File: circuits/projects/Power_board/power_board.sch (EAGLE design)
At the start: 5 parts

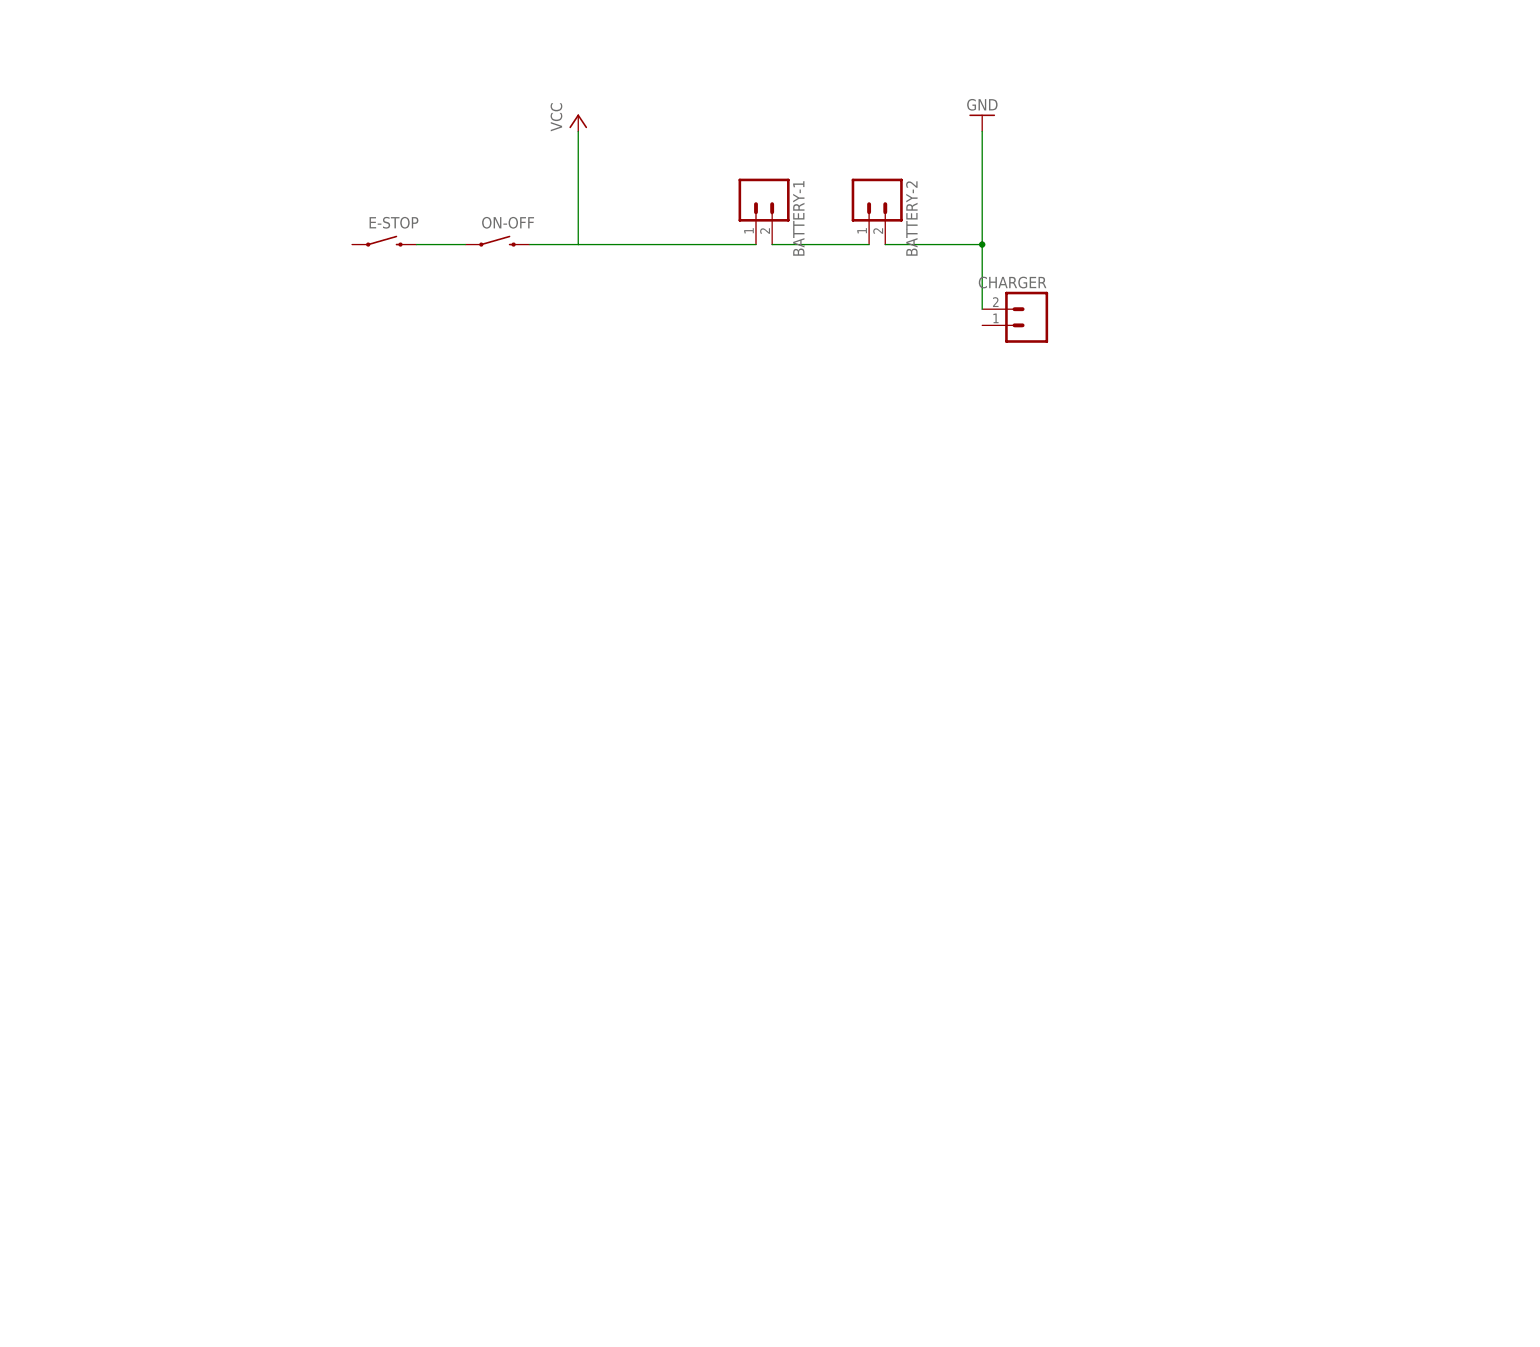
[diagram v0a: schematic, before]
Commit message: circuit board work
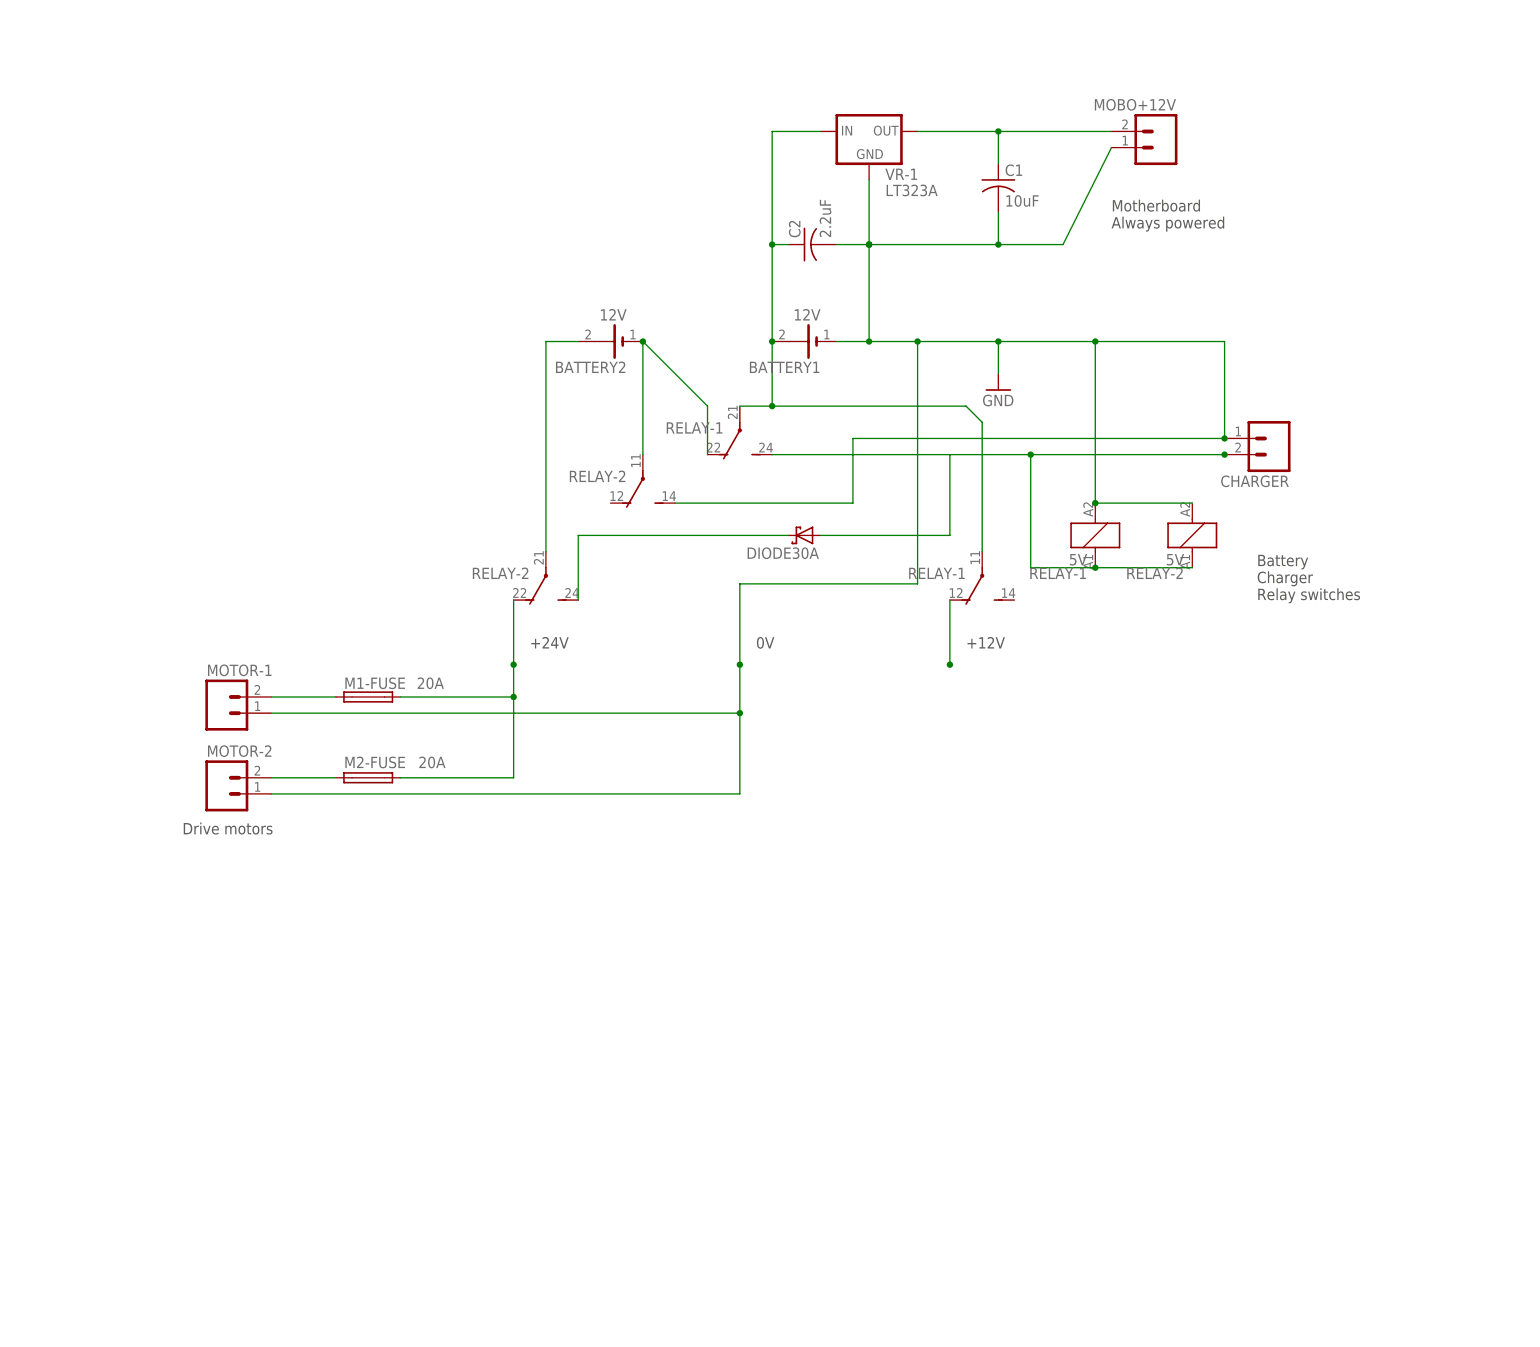
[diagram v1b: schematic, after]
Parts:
- removed BATTERY-1, BATTERY-2: (no value), iStivi - Header-Connector:M02-1.5MM
- removed E-STOP, ON-OFF: 2-PIN-SWITCH2X1.5MM_HOLES, iStivi - Button-Switch:2-PIN-SWITCH2X1.5MM_HOLES
- added BATTERY1, BATTERY2: 12V, parts:BATTERY-ST
- added C1: 10uF, parts:CAPACITOR
- added C2: 2.2uF, parts:CAPACITOR
- added DIODE30A: NTST30100SG-H, parts:NTST30100SG-H
- added M1-FUSE, M2-FUSE: 20A, parts:FUSE
- added MOBO+12V: 2-HOLESSC3.81MM, parts:2-HOLESSC3.81MM
- added MOTOR-1, MOTOR-2: 2-HOLESSC5MM, parts:2-HOLESSC5MM
- added RELAY-1, RELAY-2: 5V, parts:RT424A05
- added VR-1: LT323A, parts:LT323AT-V
- CHARGER: value (none) -> 2-HOLESSC5MM; device iStivi - Header-Connector:M02-1.5MM -> parts:2-HOLESSC5MM
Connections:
- removed net VCC: BATTERY-1.1, ON-OFF.2
- new net N$1: BATTERY1.+, C2.1, RELAY-12.P, RELAY-13.P, VR-1.IN
- new net N$10: M2-FUSE.1, MOTOR-2.2
- new net N$4: CHARGER.2, DIODE30A.A, RELAY-11.1, RELAY-13.S, RELAY-21.1
- new net N$5: BATTERY2.+, RELAY-23.P
- new net N$6: RELAY-12.O
- new net N$7: DIODE30A.C, RELAY-23.S
- new net N$8: C1.1, MOBO+12V.2, VR-1.OUT
- new net N$9: M1-FUSE.1, MOTOR-1.2
- net GND: now also BATTERY1.-, C1.2, C2.2, CHARGER.1, MOBO+12V.1, MOTOR-1.1, MOTOR-2.1, RELAY-11.2, RELAY-21.2, RELAY-22.S, VR-1.GND; no longer BATTERY-2.2, CHARGER.2
- net N$2: now also BATTERY2.-, RELAY-13.O, RELAY-22.P; no longer E-STOP.2, ON-OFF.1
- net N$3: now also M1-FUSE.2, M2-FUSE.2, RELAY-23.O; no longer BATTERY-1.2, BATTERY-2.1
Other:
- note added: "+12V"
- note added: "+24V"
- note added: "0V"
- note added: "Battery Charger Relay switches"
- note added: "Drive motors"
- note added: "Motherboard Always powered"
- moved on the sheet: CHARGER

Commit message: board work
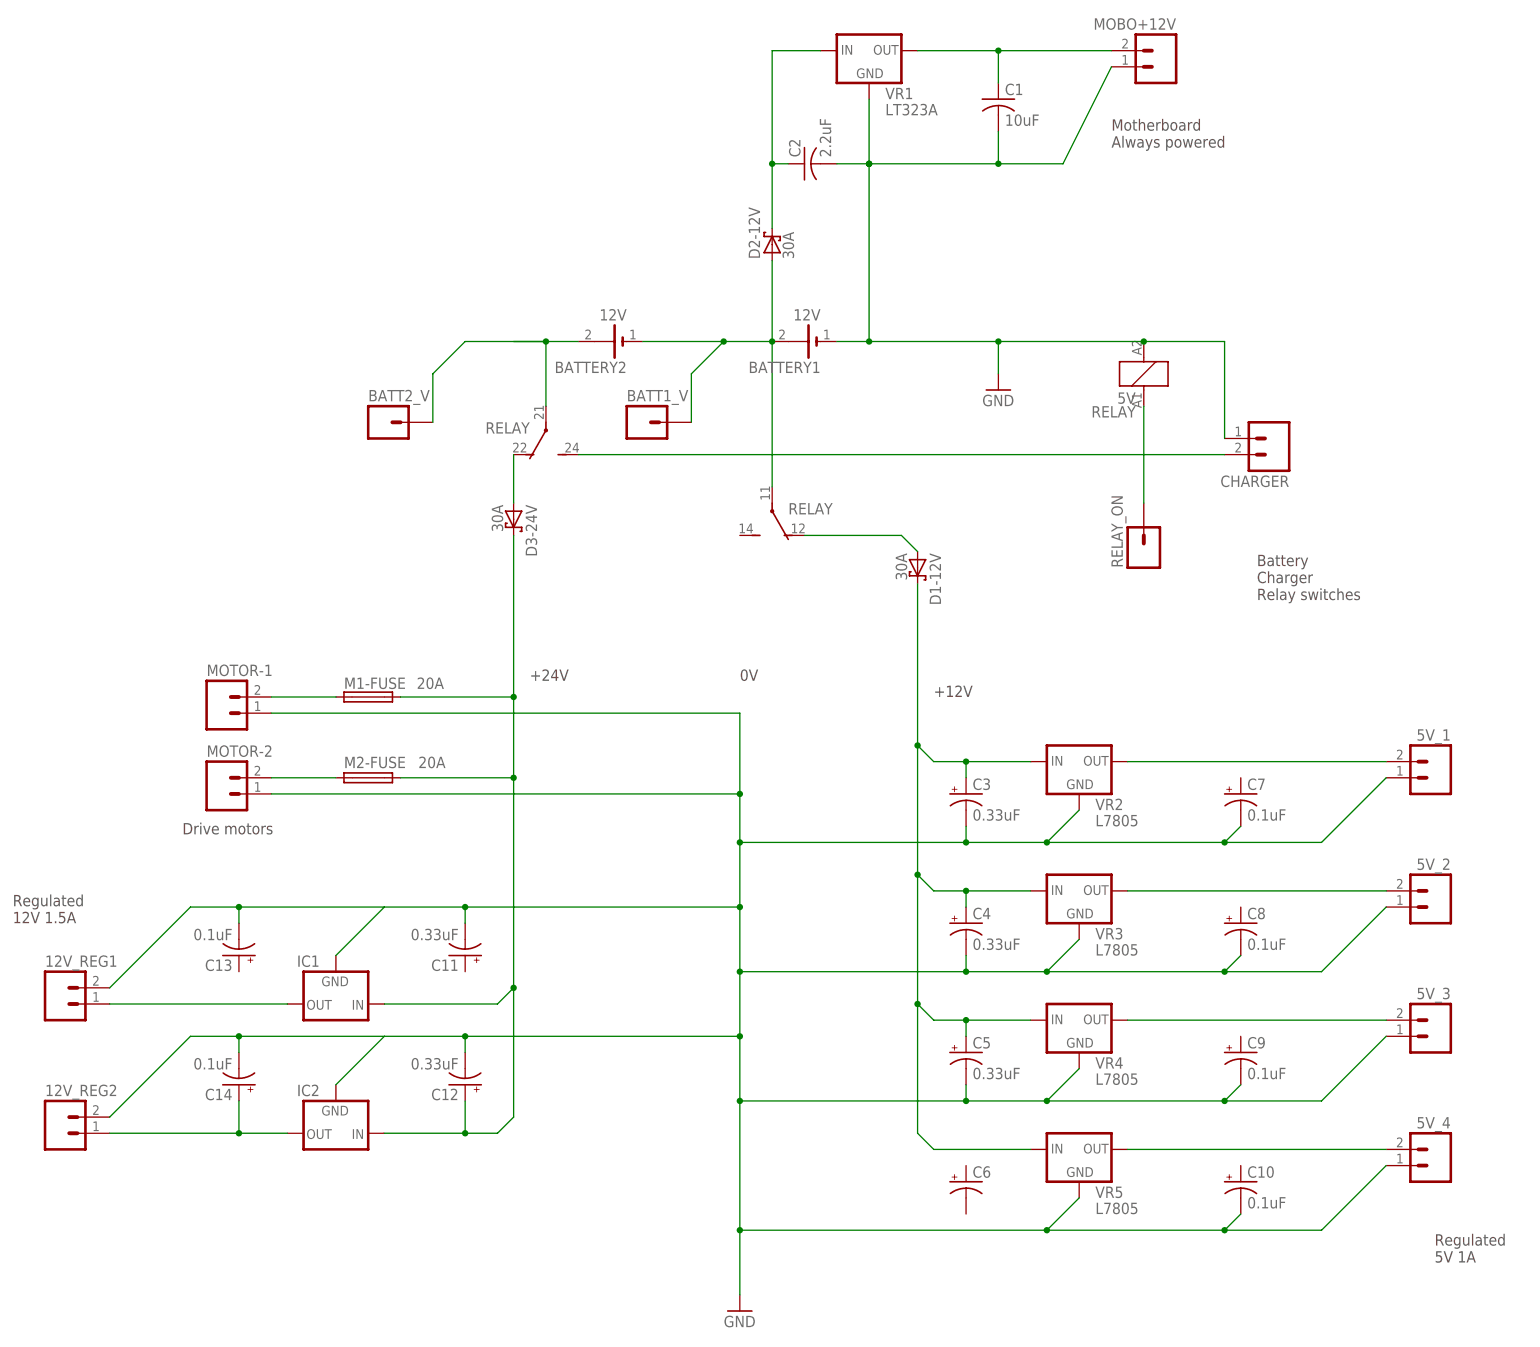
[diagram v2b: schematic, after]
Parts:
- removed DIODE30A: NTST30100SG-H, parts:NTST30100SG-H
- removed RELAY-1, RELAY-2: 5V, parts:RT424A05
- removed VR-1: LT323A, parts:LT323AT-V
- added 12V_REG1, 12V_REG2, 5V_1, 5V_2, 5V_3, 5V_4: 2-HOLESSC3.81MM, parts:2-HOLESSC3.81MM
- added BATT1_V, BATT2_V: 1-HOLE, parts:1-HOLE
- added C10, C13, C14, C7, C8, C9: 0.1uF, parts:CAPACITOR_POL
- added C11, C12, C3, C4, C5: 0.33uF, parts:CAPACITOR_POL
- added C6: (no value), parts:CAPACITOR_POL
- added D1-12V, D2-12V, D3-24V: 30A, parts:NTST30100SG-H
- added IC1, IC2: (no value), parts:L7812CD2T-TRTO-263
- added RELAY: 5V, parts:RT424A05
- added RELAY_ON: 1-HOLE", parts:1-HOLE"
- added VR1: LT323A, parts:LT323AT-V
- added VR2, VR3, VR4, VR5: L7805, parts:L7805ACD2T-TR
- CHARGER: value 2-HOLESSC5MM -> 24V
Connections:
- new net N$11: RELAY1.1, RELAY_ON.1
- new net N$12: C2.1, D2-12V.C, VR1.IN
- new net N$13: 5V_2.2, VR3.OUT
- new net N$14: 5V_3.2, VR4.OUT
- new net N$15: 5V_4.2, VR5.OUT
- new net N$16: C3.+, C4.+, C5.+, D1-12V.C, VR2.IN, VR3.IN, VR4.IN, VR5.IN
- new net N$17: 12V_REG1.1, IC1.OUT
- new net N$18: 12V_REG2.1, C14.+, IC2.OUT
- net GND: now also 12V_REG1.2, 12V_REG2.2, 5V_1.1, 5V_2.1, 5V_3.1, 5V_4.1, C10.-, C11.-, C12.-, C13.-, C14.-, C3.-, C4.-, C5.-, C7.-, C8.-, C9.-, IC1.GND, IC2.GND, RELAY1.2, VR1.GND, VR2.GND, VR3.GND, VR4.GND, VR5.GND; no longer RELAY-11.2, RELAY-21.2, RELAY-22.S, VR-1.GND
- net N$1: now also BATT1_V.1, BATTERY2.-, D2-12V.A, RELAY2.P; no longer C2.1, RELAY-12.P, RELAY-13.P, VR-1.IN
- net N$2: now also CHARGER.2, RELAY3.S; no longer BATTERY2.-, RELAY-13.O, RELAY-22.P
- net N$3: now also C12.+, D3-24V.C, IC1.IN, IC2.IN; no longer RELAY-23.O
- net N$4: now also D3-24V.A, RELAY3.O; no longer CHARGER.2, DIODE30A.A, RELAY-11.1, RELAY-13.S, RELAY-21.1
- net N$5: now also BATT2_V.1, RELAY3.P; no longer RELAY-23.P
- net N$6: now also D1-12V.A, RELAY2.O; no longer RELAY-12.O
- net N$7: now also 5V_1.2, VR2.OUT; no longer DIODE30A.C, RELAY-23.S
- net N$8: now also VR1.OUT; no longer VR-1.OUT
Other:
- note added: "Regulated 12V 1.5A"
- note added: "Regulated 5V 1A"
- moved on the sheet: C1, C2, MOBO+12V
